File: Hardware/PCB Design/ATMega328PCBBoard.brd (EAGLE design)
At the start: 38.1 x 16.5 mm, 12 parts

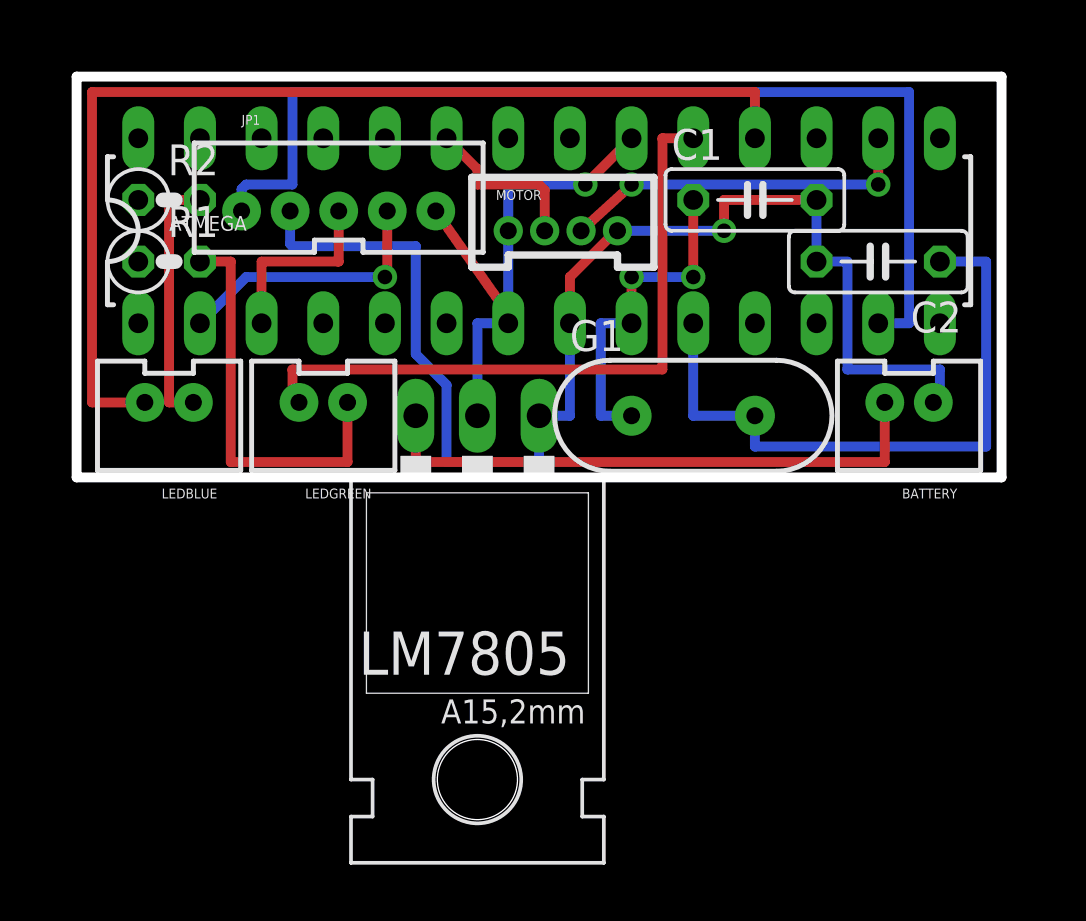
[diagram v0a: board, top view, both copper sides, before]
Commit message: updated pcb
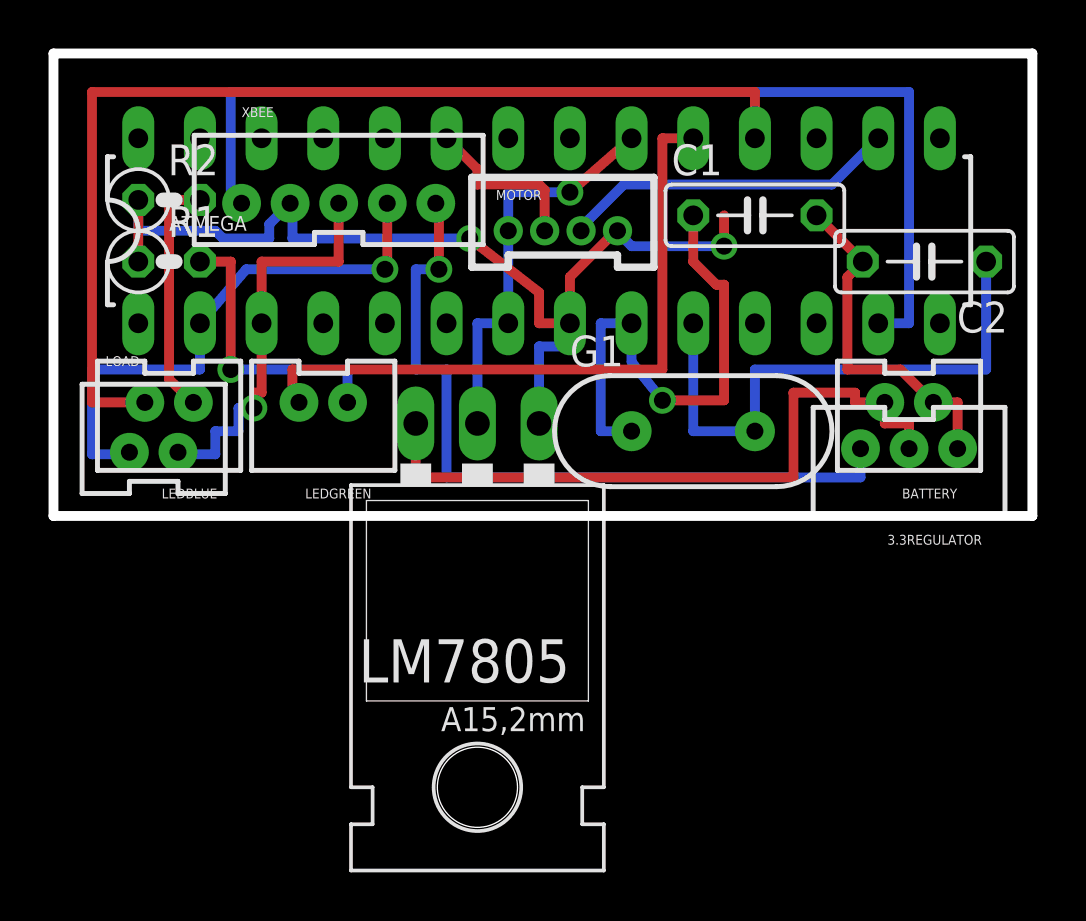
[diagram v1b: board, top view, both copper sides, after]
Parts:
- removed JP1: (no value), SparkFun-Connectors:JST-5-PTH-VERT
- added 3.3REGULATOR: (no value), SparkFun-Connectors:JST-3-PTH-VERT
- added LOAD: (no value), SparkFun-Connectors:JST-2-PTH-VERT
- added XBEE: (no value), SparkFun-Connectors:JST-5-PTH-VERT
- moved C2 1.91 mm to (92.1, 44.5)
- moved C1 0.64 mm to (85.1, 46.4)
- moved G1 0.63 mm to (82.5, 37.5)
- moved LM7805 0.32 mm to (73.7, 34.0)
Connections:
- removed net N$6: R1.1
- removed net N$7: R2.1
- removed net XBEE2: ATMEGA.8, BATTERY.1, C1.2, C2.2, JP1.2, LM7805.IN, MOTOR.4
- new net 3VCC: 3.3REGULATOR.3, XBEE.5
- new net GND: 3.3REGULATOR.1, ATMEGA.8, BATTERY.1, C1.2, C2.2, LM7805.IN, MOTOR.4, R1.1, R2.1, XBEE.2
- net 0: now also LOAD.1, XBEE.4; no longer JP1.4
- net 1: now also LOAD.2, XBEE.3; no longer JP1.3
- net 7: now also XBEE.1; no longer JP1.1
- net N$4: now also 3.3REGULATOR.2
- net VCC: no longer JP1.5
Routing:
- net GND: track 0.00 -> 56.6 mm, vias 0 -> 2
- net XBEE2: track 54.6 -> 0.00 mm, vias 1 -> 0
- net 3VCC: track 0.00 -> 31.9 mm, vias 0 -> 1
- net 0: track 11.2 -> 22.8 mm
- net 1: track 7.80 -> 17.0 mm, vias 0 -> 1
- net N$2: track 14.0 -> 21.5 mm, vias 2 -> 1
- net VCC: track 22.2 -> 16.7 mm
- net N$3: track 16.8 -> 11.9 mm, vias 0 -> 1
- net N$4: track 23.7 -> 28.3 mm
- net N$1: track 26.7 -> 23.5 mm
- net 10: track 14.9 -> 13.9 mm, vias 2 -> 0
- net 7: track 43.1 -> 43.7 mm
- net N$5: track 10.6 -> 10.0 mm
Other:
- board size 38.1 x 16.5 mm -> 40.3 x 19.1 mm
